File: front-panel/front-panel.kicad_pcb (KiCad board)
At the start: 2 copper layers, 87 x 326.5 mm, 21 parts

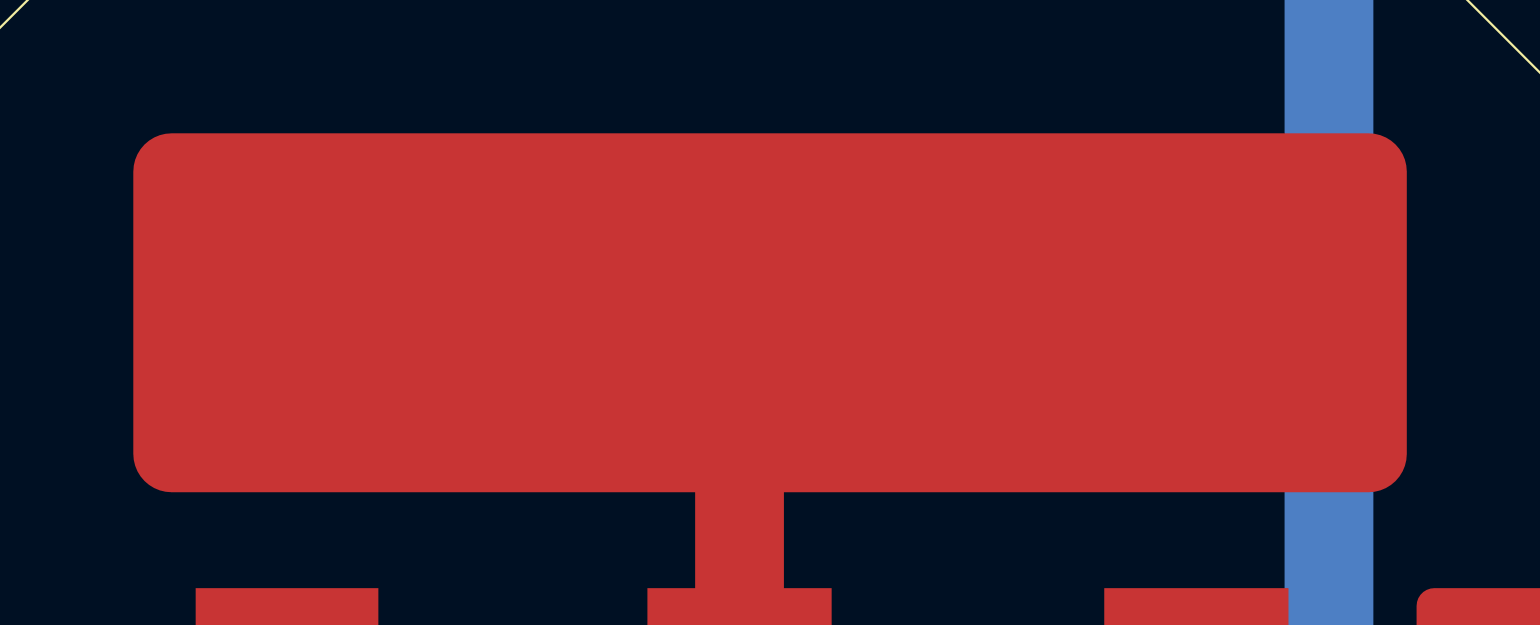
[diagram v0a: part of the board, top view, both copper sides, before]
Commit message: reviewed boards
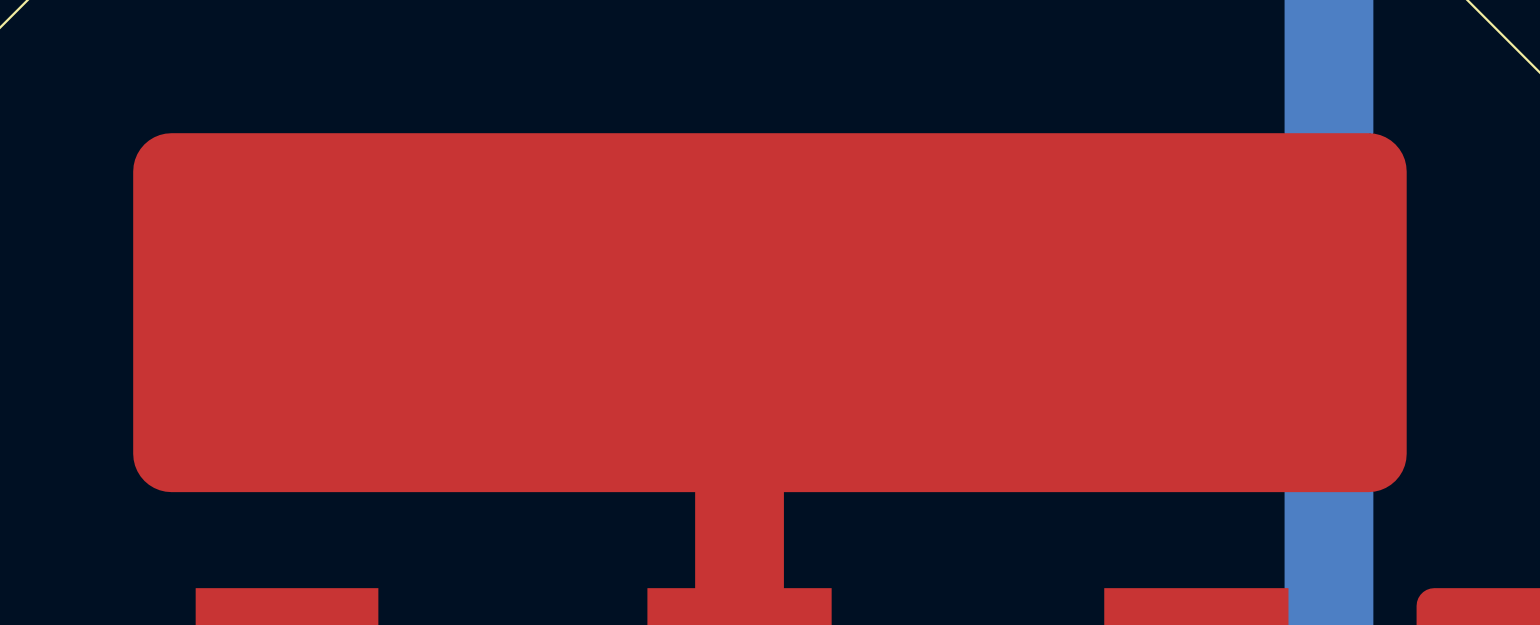
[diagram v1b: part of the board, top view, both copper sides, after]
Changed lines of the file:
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@@
 		)
 		(fp_line
-			(start -10.45 33.1)
-			(end 3.55 47.35)
-			(stroke
-				(width 0.1)
-				(type solid)
-			)
-			(layer "F.CrtYd")
-		)
-		(fp_line
 			(start -10.43 33.03)
 			(end 3.57 47.28)
@@
 		)
 		(fp_line
-			(start -10.45 33.1)
-			(end 3.55 47.35)
-			(stroke
-				(width 0.1)
-				(type solid)
-			)
-			(layer "F.CrtYd")
-		)
-		(fp_line
 			(start -10.43 33.03)
 			(end 3.57 47.28)
@@
 		(sheetfile "front-panel.kicad_sch")
 		(attr smd)
+		(fp_poly
+			(pts
+				(xy -26.655 12.105) (xy -12.66 12.105) (xy -12.66 26.057802)
+			)
+			(stroke
+				(width 0)
+				(type solid)
+			)
+			(fill yes)
+			(layer "F.Mask")
+		)
 		(fp_line
 			(start -12.74 26.17)
@@
 			)
 		)
+		(pad "" smd rect
+			(at -19.6575 -20.815)
+			(size 65.84 13.995)
+			(layers "F.Mask")
+		)
+		(pad "" smd rect
+			(at 0.2375 -13.838599)
+			(size 79.792802 25.795)
+			(layers "F.Mask")
+		)
 		(pad "1" smd rect
 			(at -31.3 -12.915 270)
@@
 		)
 		(pad "2" smd roundrect
-			(at -6.925 -15.545 270)
+			(at -6.93 -15.54 270)
 			(size 16.17 57.37)
 			(layers "F.Cu" "F.Mask" "F.Paste")
@@
 			(pinfunction "-")
 			(pintype "passive")
-			(clearance 0)
 		)
 		(embedded_fonts no)
@@
 	)
 	(zone
-		(net 0)
-		(net_name "")
-		(layer "F.Mask")
-		(hatch edge 0.5)
-		(connect_pads
-			(clearance 0.5)
-		)
-		(min_thickness 0.25)
-		(filled_areas_thickness no)
-		(fill yes
-			(thermal_gap 0.5)
-			(thermal_bridge_width 0.5)
-		)
-		(polygon
-			(pts
-				(xy 107.89 80.36) (xy 107.89 54.36) (xy 121.89 40.36) (xy 187.88 40.37) (xy 187.88 80.37)
-			)
-		)
-	)
-	(zone
